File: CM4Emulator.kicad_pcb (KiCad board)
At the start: 2 copper layers, 4 parts, among them U1 Compute_Module_4_Functional, U2 TFP401APZP, U3 WM8960CGEFL/RV

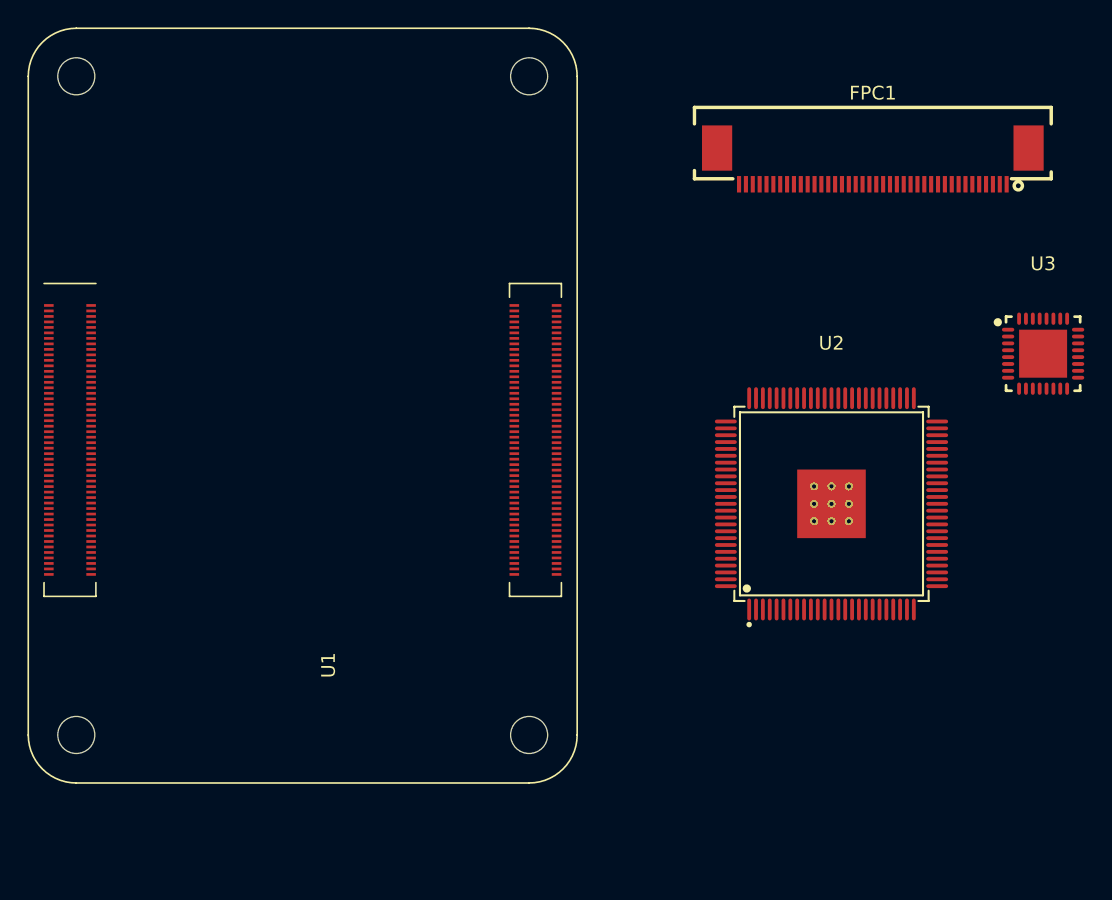
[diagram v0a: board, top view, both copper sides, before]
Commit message: added display things + others
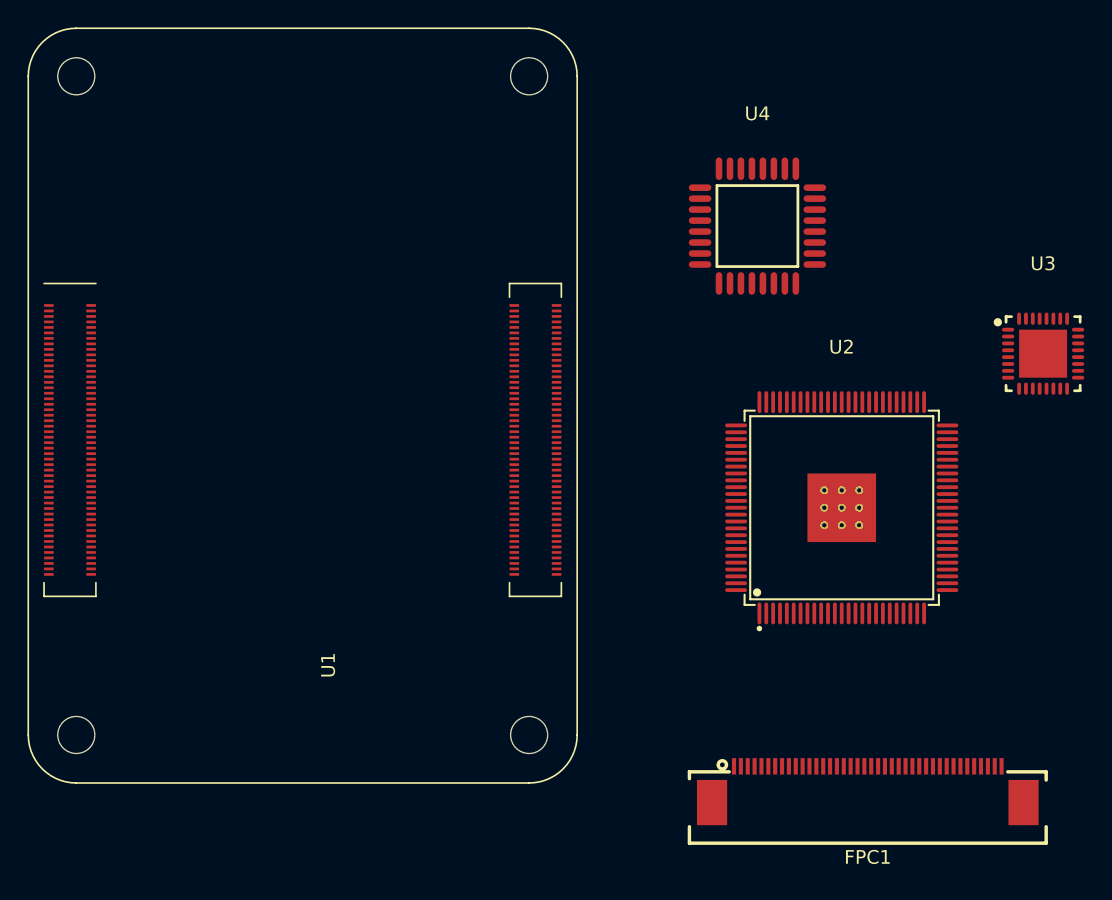
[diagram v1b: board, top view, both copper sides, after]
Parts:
- added U4: TUSB2046BVFR, easyeda2kicad:LQFP-32_L7.0-W7.0-P0.80-LS9.0-TL, F.Cu at (182.4, 74.5)
- moved FPC1 45.1 mm to (190.4, 115.2), turned to 180 degrees
- moved U2 0.80 mm to (188.5, 95.1)
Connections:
- FPC1 pad 1: unconnected-(FPC1-Pad1) -> /Display/LEDK
- FPC1 pad 10: unconnected-(FPC1-Pad10) -> /Display/R5
- FPC1 pad 11: unconnected-(FPC1-Pad11) -> /Display/R6
- FPC1 pad 12: unconnected-(FPC1-Pad12) -> /Display/R7
- FPC1 pad 13: unconnected-(FPC1-Pad13) -> /Display/G0
- FPC1 pad 14: unconnected-(FPC1-Pad14) -> /Display/G1
- FPC1 pad 15: unconnected-(FPC1-Pad15) -> /Display/G2
- FPC1 pad 16: unconnected-(FPC1-Pad16) -> /Display/G3
- FPC1 pad 17: unconnected-(FPC1-Pad17) -> /Display/G4
- FPC1 pad 18: unconnected-(FPC1-Pad18) -> /Display/G5
- FPC1 pad 19: unconnected-(FPC1-Pad19) -> /Display/G6
- FPC1 pad 2: unconnected-(FPC1-Pad2) -> +24V
- FPC1 pad 20: unconnected-(FPC1-Pad20) -> /Display/G7
- FPC1 pad 21: unconnected-(FPC1-Pad21) -> /Display/B0
- FPC1 pad 22: unconnected-(FPC1-Pad22) -> /Display/B1
- FPC1 pad 23: unconnected-(FPC1-Pad23) -> /Display/B2
- FPC1 pad 24: unconnected-(FPC1-Pad24) -> /Display/B3
- FPC1 pad 25: unconnected-(FPC1-Pad25) -> /Display/B4
- FPC1 pad 26: unconnected-(FPC1-Pad26) -> /Display/B5
- FPC1 pad 27: unconnected-(FPC1-Pad27) -> /Display/B6
- FPC1 pad 28: unconnected-(FPC1-Pad28) -> /Display/B7
- FPC1 pad 29: unconnected-(FPC1-Pad29) -> GND
- FPC1 pad 3: unconnected-(FPC1-Pad3) -> GND
- FPC1 pad 30: unconnected-(FPC1-Pad30) -> /Display/CLK
- FPC1 pad 31: unconnected-(FPC1-Pad31) -> /Display/ON/OFF
- FPC1 pad 32: unconnected-(FPC1-Pad32) -> /Display/HSYNC
- FPC1 pad 33: unconnected-(FPC1-Pad33) -> /Display/VSYNC
- FPC1 pad 34: unconnected-(FPC1-Pad34) -> /Display/DE
- FPC1 pad 36: unconnected-(FPC1-Pad36) -> GND
- FPC1 pad 4: unconnected-(FPC1-Pad4) -> VDD
- FPC1 pad 5: unconnected-(FPC1-Pad5) -> /Display/R0
- FPC1 pad 6: unconnected-(FPC1-Pad6) -> /Display/R1
- FPC1 pad 7: unconnected-(FPC1-Pad7) -> /Display/R2
- FPC1 pad 8: unconnected-(FPC1-Pad8) -> /Display/R3
- FPC1 pad 9: unconnected-(FPC1-Pad9) -> /Display/R4
- U1 pad 103: unconnected-(U1D-USB_N-Pad103) -> Net-(U1D-USB_N)
- U1 pad 105: unconnected-(U1D-USB_P-Pad105) -> Net-(U1D-USB_P)
- U2 pad 10: unconnected-(U2-QE0-Pad10) -> /Display/B0
- U2 pad 11: unconnected-(U2-QE1-Pad11) -> /Display/B1
- U2 pad 12: unconnected-(U2-QE2-Pad12) -> /Display/B2
- U2 pad 13: unconnected-(U2-QE3-Pad13) -> /Display/B3
- U2 pad 14: unconnected-(U2-QE4-Pad14) -> /Display/B4
- U2 pad 15: unconnected-(U2-QE5-Pad15) -> /Display/B5
- U2 pad 16: unconnected-(U2-QE6-Pad16) -> /Display/B6
- U2 pad 17: unconnected-(U2-QE7-Pad17) -> /Display/B7
- U2 pad 20: unconnected-(U2-QE8-Pad20) -> /Display/G0
- U2 pad 21: unconnected-(U2-QE9-Pad21) -> /Display/G1
- U2 pad 22: unconnected-(U2-QE10-Pad22) -> /Display/G2
- U2 pad 23: unconnected-(U2-QE11-Pad23) -> /Display/G3
- U2 pad 24: unconnected-(U2-QE12-Pad24) -> /Display/G4
- U2 pad 25: unconnected-(U2-QE13-Pad25) -> /Display/G5
- U2 pad 26: unconnected-(U2-QE14-Pad26) -> /Display/G6
- U2 pad 27: unconnected-(U2-QE15-Pad27) -> /Display/G7
- U2 pad 30: unconnected-(U2-QE16-Pad30) -> /Display/R0
- U2 pad 31: unconnected-(U2-QE17-Pad31) -> /Display/R1
- U2 pad 32: unconnected-(U2-QE18-Pad32) -> /Display/R2
- U2 pad 33: unconnected-(U2-QE19-Pad33) -> /Display/R3
- U2 pad 34: unconnected-(U2-QE20-Pad34) -> /Display/R4
- U2 pad 35: unconnected-(U2-QE21-Pad35) -> /Display/R5
- U2 pad 36: unconnected-(U2-QE22-Pad36) -> /Display/R6
- U2 pad 37: unconnected-(U2-QE23-Pad37) -> /Display/R7
